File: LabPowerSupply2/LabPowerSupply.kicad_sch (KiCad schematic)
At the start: 2 parts

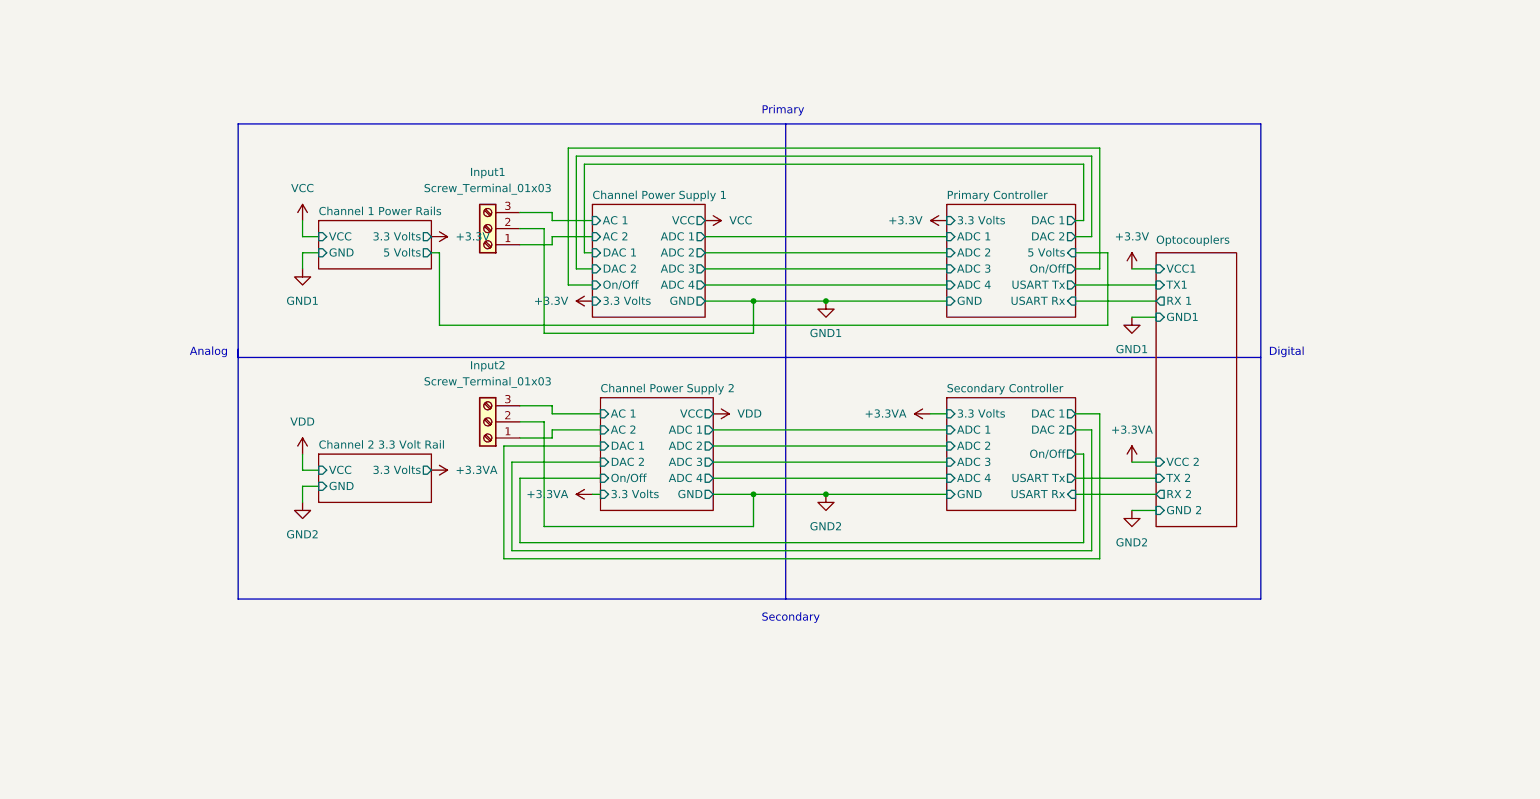
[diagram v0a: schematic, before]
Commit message: Beautifing the Schematic
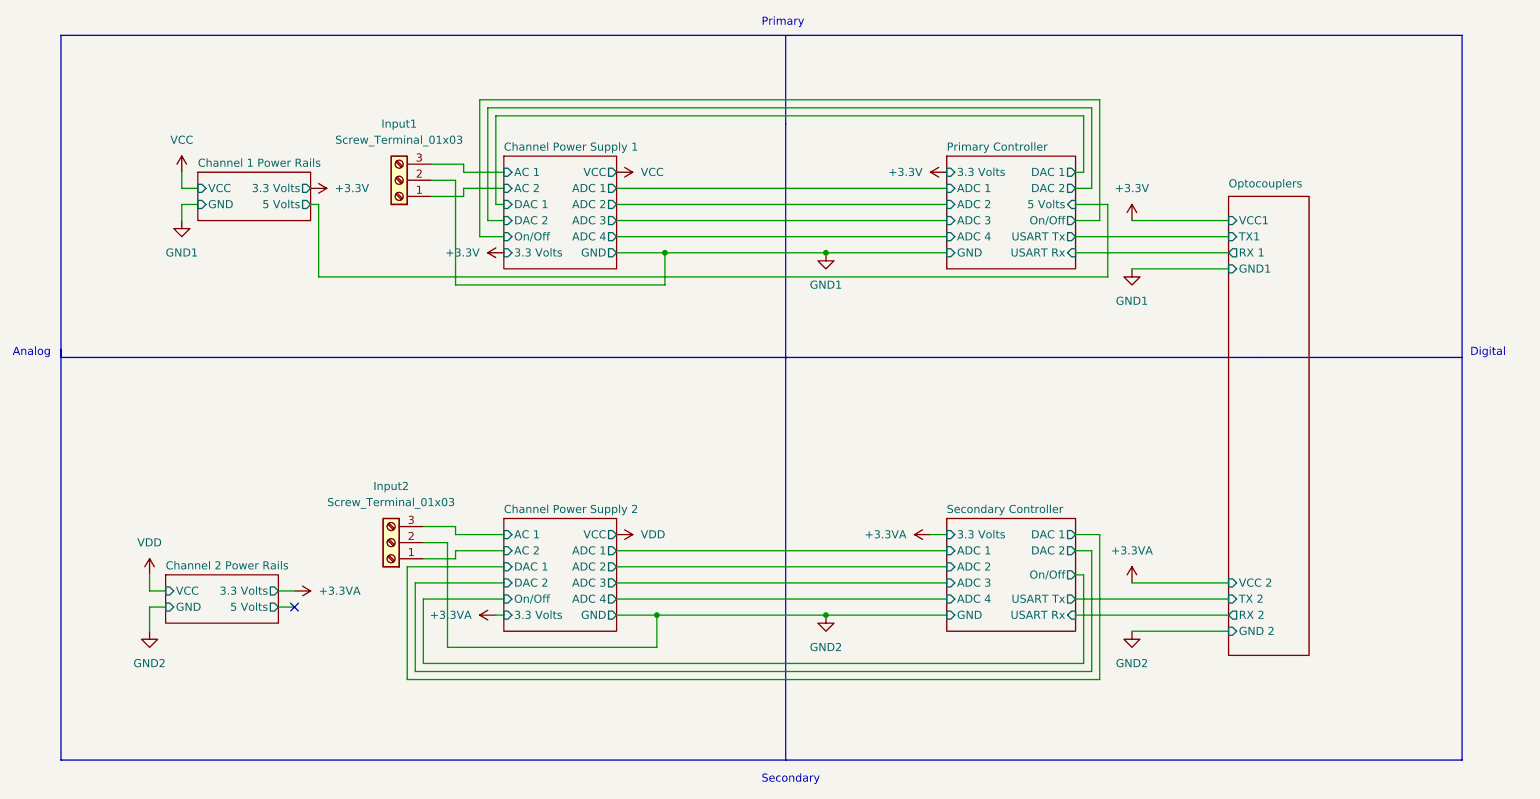
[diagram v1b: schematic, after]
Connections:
- no-connect marks 0 -> 1
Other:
- removed sheet Channel 2 3.3 Volt Rail
- added sheet Channel 2 Power Rails (Channel1PowerRails.kicad_sch)
- moved on the sheet: Input1, Input2

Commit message: Changed symbols to actual MOSFETs
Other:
- sheet Channel 1 Power Rails: file Channel1PowerRails.kicad_sch -> PowerRails.kicad_sch
- sheet Channel 2 Power Rails: file Channel1PowerRails.kicad_sch -> PowerRails.kicad_sch
